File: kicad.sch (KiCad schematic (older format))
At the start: 31 parts, among them J1 Screw_Terminal_01x03, J2 Screw_Terminal_01x03, J3 Conn_01x03_Male, J4 Conn_01x03_Male, J5 Conn_01x03_Male, J6 Conn_01x06_Male, K1 SANYOU_SRD_Form_C, K2 SANYOU_SRD_Form_C, Q1 BC817, Q2 BC817, Q3 BC817, Q4 IRF540N, Q5 BC817, U1 ESP32_DevKit_V1_DOIT, U2 4N25, U3 4N25, U4 4N25, U5 4N25

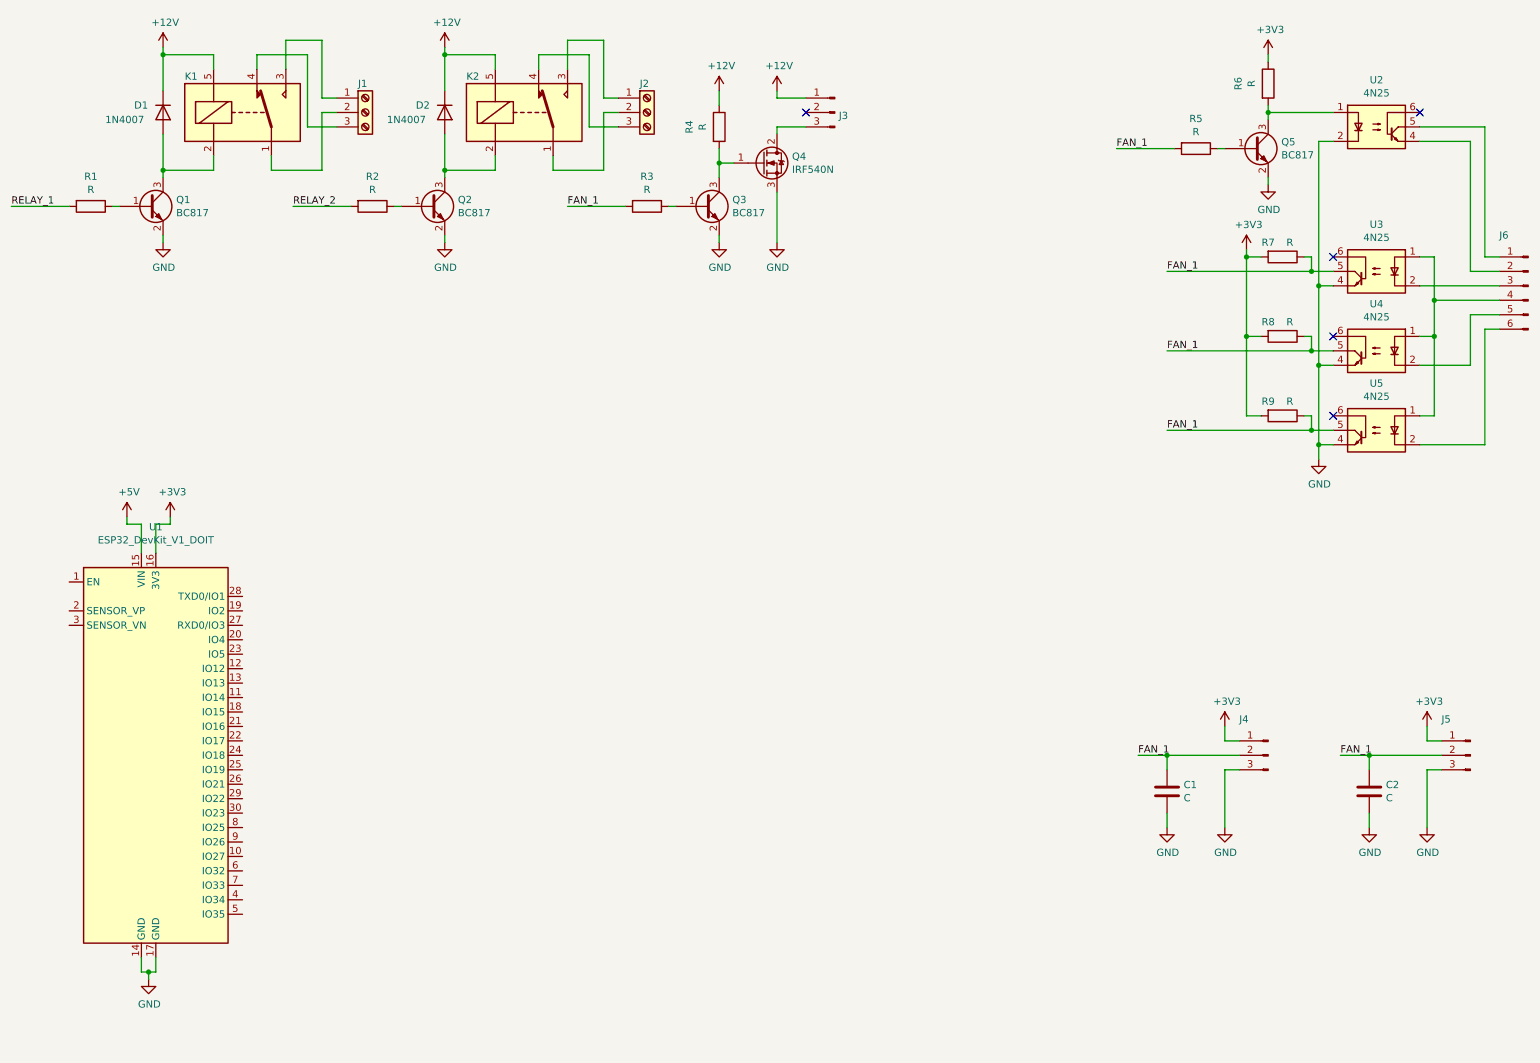
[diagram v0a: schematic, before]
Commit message: several changes
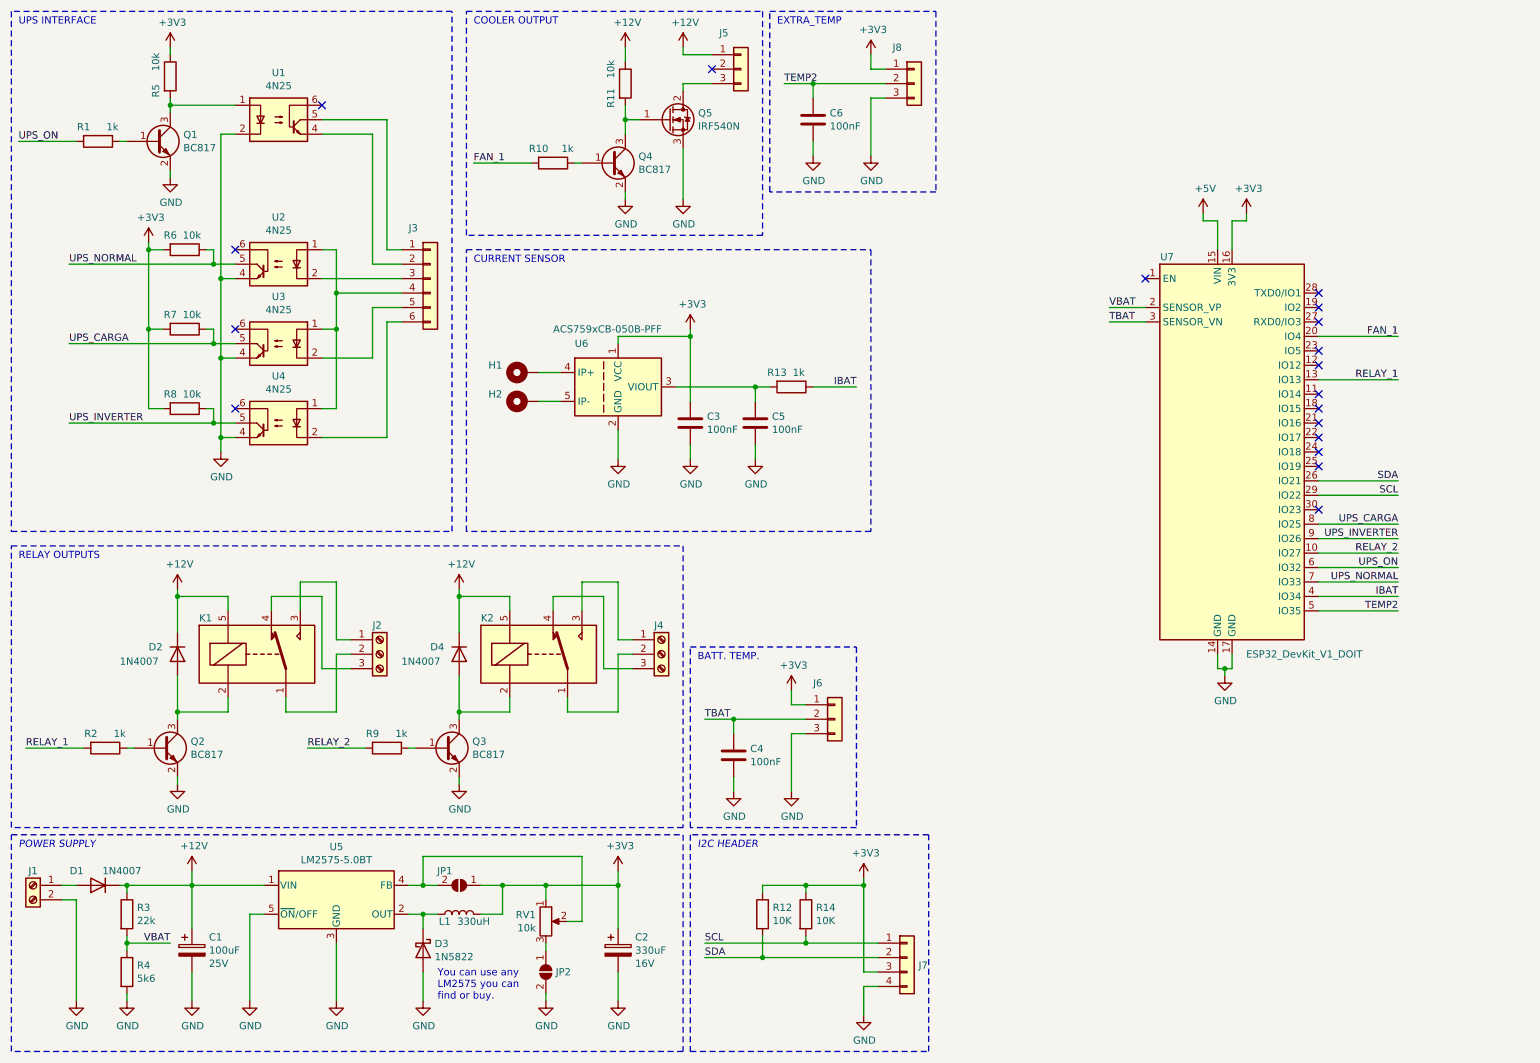
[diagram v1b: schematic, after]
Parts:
- removed C2: C, symbol Device:C
- removed J3, J4, J5: Conn_01x03_Male, symbol Connector:Conn_01x03_Male
- removed J6: Conn_01x06_Male, symbol Connector:Conn_01x06_Male
- added C1: 100uF, symbol Device:CP
- added C2: 330uF, symbol Device:CP
- added C3, C5, C6: 100nF, Capacitor_SMD:C_1206_3216Metric_Pad1.33x1.80mm_HandSolder, symbol Device:C
- added D1: 1N4007, Diode_THT:D_DO-41_SOD81_P7.62mm_Horizontal, symbol Diode:1N4007
- added D3: 1N5822, Diode_THT:D_DO-201_P12.70mm_Horizontal, symbol Diode:1N5822
- added H1, H2: MountingHole_Pad, symbol Mechanical:MountingHole_Pad
- added J1: Screw_Terminal_01x02, TerminalBlock:TerminalBlock_bornier-2_P5.08mm, symbol Connector:Screw_Terminal_01x02
- added J3: Conn_01x06, symbol Connector_Generic:Conn_01x06
- added J5, J6, J8: Conn_01x03, symbol Connector_Generic:Conn_01x03
- added J7: Conn_01x04, symbol Connector_Generic:Conn_01x04
- added JP1, JP2: SolderJumper_2_Open, symbol Jumper:SolderJumper_2_Open
- added L1: 330uH, symbol Device:L
- added R12, R14: 10K, Resistor_SMD:R_1206_3216Metric_Pad1.30x1.75mm_HandSolder, symbol Device:R
- added R13: 1k, Resistor_SMD:R_1206_3216Metric_Pad1.30x1.75mm_HandSolder, symbol Device:R
- added R3: 22k, Resistor_SMD:R_0805_2012Metric_Pad1.20x1.40mm_HandSolder, symbol Device:R
- added R4: 5k6, Resistor_SMD:R_0805_2012Metric_Pad1.20x1.40mm_HandSolder, symbol Device:R
- added RV1: 10k, Resistor_SMD:R_1206_3216Metric_Pad1.30x1.75mm_HandSolder, symbol Device:R_POT
- added U5: LM2575-5.0BT, Package_TO_SOT_THT:TO-220-5_Vertical, symbol Regulator_Switching:LM2575-5.0BT
- added U6: ACS759xCB-050B-PFF, Sensor_Current:Allegro_CB_PFF, symbol Sensor_Current:ACS759xCB-050B-PFF
- C4: renamed from C1; value C -> 100nF; footprint (none) -> Capacitor_SMD:C_1206_3216Metric_Pad1.33x1.80mm_HandSolder
- D2: renamed from D1; footprint Diode_THT:D_DO-41_SOD81_P10.16mm_Horizontal -> Diode_THT:D_DO-41_SOD81_P7.62mm_Horizontal
- D4: renamed from D2; footprint Diode_THT:D_DO-41_SOD81_P10.16mm_Horizontal -> Diode_THT:D_DO-41_SOD81_P7.62mm_Horizontal
- J2: renamed from J1; footprint (none) -> TerminalBlock:TerminalBlock_bornier-3_P5.08mm
- J4: renamed from J2; footprint (none) -> TerminalBlock:TerminalBlock_bornier-3_P5.08mm
- R1: renamed from R5; value R -> 1k; footprint (none) -> Resistor_SMD:R_1206_3216Metric_Pad1.30x1.75mm_HandSolder
- R10: renamed from R3; value R -> 1k; footprint (none) -> Resistor_SMD:R_1206_3216Metric_Pad1.30x1.75mm_HandSolder
- R11: renamed from R4; value R -> 10k; footprint (none) -> Resistor_SMD:R_1206_3216Metric_Pad1.30x1.75mm_HandSolder
- R2: renamed from R1; value R -> 1k; footprint (none) -> Resistor_SMD:R_1206_3216Metric_Pad1.30x1.75mm_HandSolder
- R5: renamed from R6; value R -> 10k; footprint (none) -> Resistor_SMD:R_1206_3216Metric_Pad1.30x1.75mm_HandSolder
- R6: renamed from R7; value R -> 10k; footprint (none) -> Resistor_SMD:R_1206_3216Metric_Pad1.30x1.75mm_HandSolder
- R7: renamed from R8; value R -> 10k; footprint (none) -> Resistor_SMD:R_1206_3216Metric_Pad1.30x1.75mm_HandSolder
- R8: renamed from R9; value R -> 10k; footprint (none) -> Resistor_SMD:R_1206_3216Metric_Pad1.30x1.75mm_HandSolder
- R9: renamed from R2; value R -> 1k; footprint (none) -> Resistor_SMD:R_1206_3216Metric_Pad1.30x1.75mm_HandSolder
- renumbered Q5 to Q1, Q1 to Q2, Q2 to Q3, Q3 to Q4, Q4 to Q5, U2 to U1, U3 to U2, U4 to U3, U5 to U4, U1 to U7
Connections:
- net +12V: now also C1.1, D1.1 (K), J5.1 (Pin_1), R3.1, U5.1 (VIN)
- net +3V3: now also C2.1, C3.1, J6.1 (Pin_1), J7.3 (Pin_3), J8.1 (Pin_1), JP1.1 (A), L1.2, R12.1, R14.1, RV1.1, U6.1 (VCC)
- net FAN_1: now also U7.20 (IO4); no longer C4.1, R1.2, R6.1, R7.1, R8.1, U2.5, U3.5, U4.5
- net GND: now also C1.2, C2.2, C3.2, C5.2, C6.2, D3.2 (A), J1.2 (Pin_2), J6.3 (Pin_3), J7.4 (Pin_4), J8.3 (Pin_3), JP2.2 (B), R4.2, U5.3 (GND), U5.5 (~ON~/OFF), U6.2 (GND)
- net RELAY_1: now also U7.13 (IO13)
- net RELAY_2: now also U7.10 (IO27)
- net VBAT: now reaches U7.2 (SENSOR_VP)
- net VBAT: now also R3.2, R4.1
- net SDA: now reaches U7.26 (IO21)
- net SDA: now also J7.2 (Pin_2), R12.2
- net SCL: now reaches U7.29 (IO22)
- net SCL: now also J7.1 (Pin_1), R14.2
- net TBAT: now reaches U7.3 (SENSOR_VN)
- net TBAT: now also C4.1, J6.2 (Pin_2)
- net IBAT: now reaches U7.4 (IO34)
- net IBAT: now also R13.1
- net TEMP2: now reaches U7.5 (IO35)
- net TEMP2: now also C6.1, J8.2 (Pin_2)
- net UPS_ON: now reaches U7.6 (IO32)
- net UPS_ON: now also R1.2
- net UPS_NORMAL: now reaches U7.7 (IO33)
- net UPS_NORMAL: now also R6.1, U2.5
- net UPS_CARGA: now reaches U7.8 (IO25)
- net UPS_CARGA: now also R7.1, U3.5
- net UPS_INVERTER: now reaches U7.9 (IO26)
- net UPS_INVERTER: now also R8.1, U4.5
- net at U1.4: now also J3.2 (Pin_2)
- net at U1.5: now also J3.1 (Pin_1)
- net at Q5.2 (D): now also J5.3 (Pin_3)
- net at U2.1, U3.1, U4.1: now also J3.4 (Pin_4)
- net at U2.2: now also J3.3 (Pin_3)
- net at U3.2: now also J3.5 (Pin_5)
- net at U4.2: now also J3.6 (Pin_6)
- new net: D3.1 (K), L1.1, U5.2 (OUT)
- new net: JP1.2 (B), RV1.2, U5.4 (FB)
- new net: D1.2 (A), J1.1 (Pin_1)
- new net: C5.1, R13.2, U6.3 (VIOUT)
- new net: H1.1, U6.4 (IP+)
- new net: H2.1, U6.5 (IP-)
- new net: JP2.1 (A), RV1.3
- no-connect marks 5 -> 18
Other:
- note added: "BATT. TEMP."
- note added: "COOLER OUTPUT"
- note added: "CURRENT SENSOR"
- note added: "EXTRA_TEMP"
- note added: "I2C HEADER"
- note added: "POWER SUPPLY"
- note added: "RELAY OUTPUTS"
- note added: "UPS INTERFACE"
- note added: "You can use any\nLM2575 you can\nfind or buy."
- moved on the sheet: C4, D2, D4, J2, J4, K1, K2, Q1, Q2, Q3, Q4, Q5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
